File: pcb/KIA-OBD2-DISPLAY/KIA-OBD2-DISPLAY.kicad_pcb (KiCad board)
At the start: 2 copper layers, 132.1 x 19 mm, 13 parts, among them J1 Conn_01x07_Pin, U10 MCP2515-xST, U11 MCP2515-xST, U4 CAP1188-1-CP-TR, U6 TJA1050, U7 TJA1050, U9 ESP32-C6-MINI-1/U, Y1 Crystal_GND24_Small, Y4 Crystal_GND24_Small

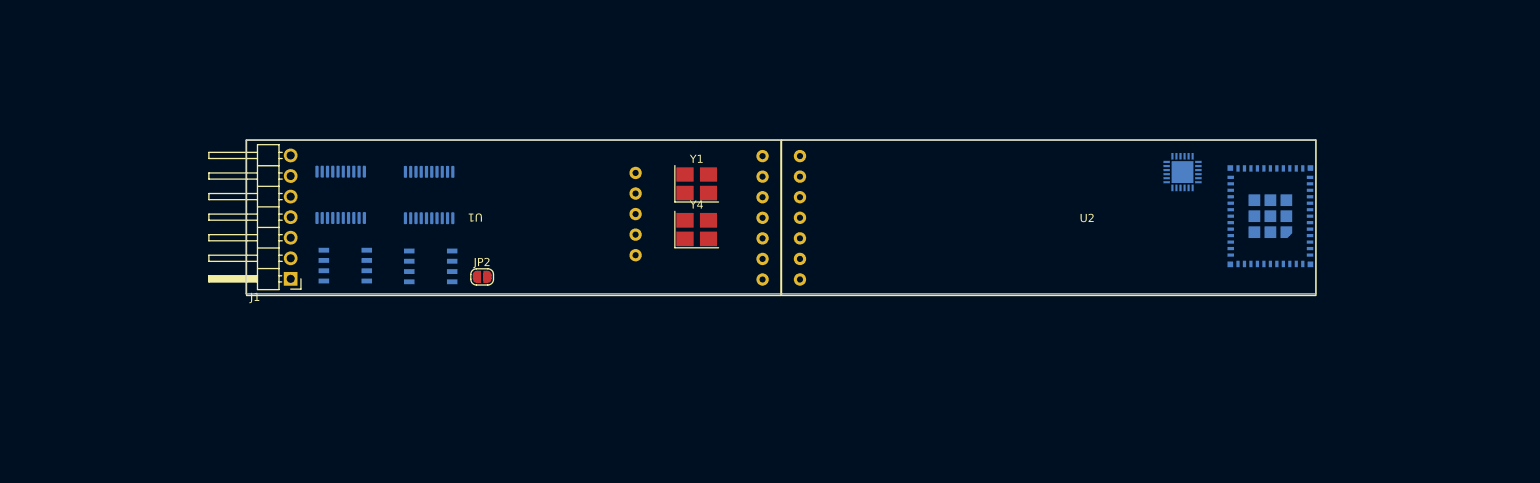
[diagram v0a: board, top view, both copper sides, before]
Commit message: pcb work
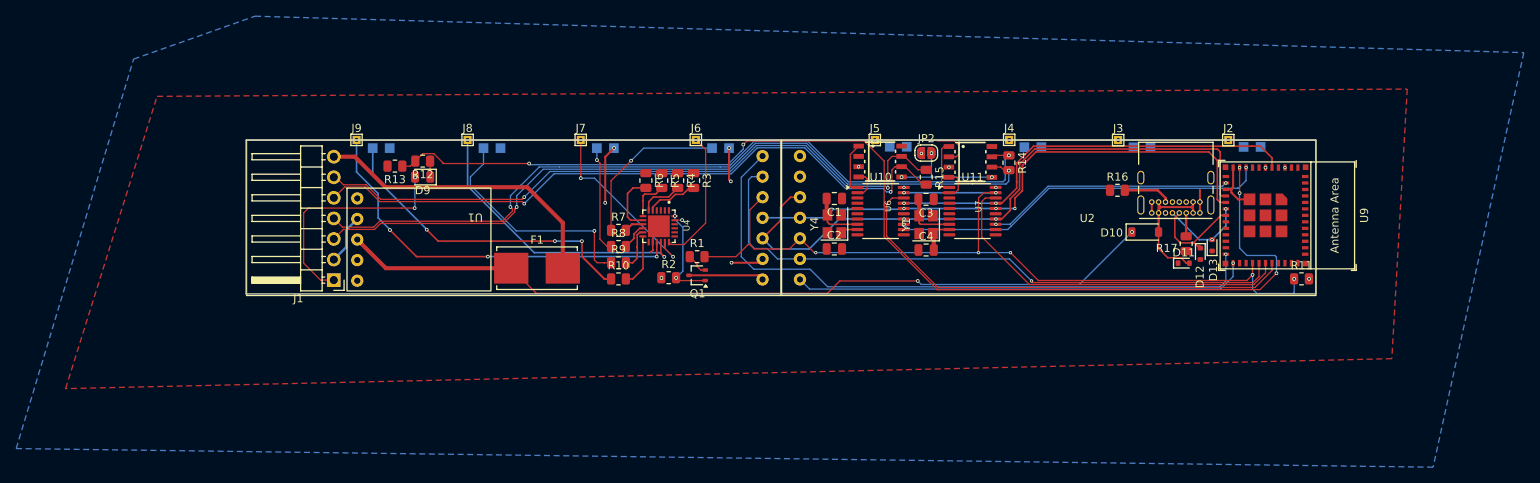
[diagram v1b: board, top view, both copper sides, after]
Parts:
- added C1: 22pF, Capacitor_SMD:C_0805_2012Metric, F.Cu at (165.9, 85.2)
- added C2: 22pF, Capacitor_SMD:C_0805_2012Metric, F.Cu at (165.9, 91.5)
- added C3: 22pF, Capacitor_SMD:C_0805_2012Metric, F.Cu at (177.3, 85.3)
- added C4: 22pF, Capacitor_SMD:C_0805_2012Metric, F.Cu at (177.3, 91.6)
- added D1: LED, LED_0602:LED_QBLP617-IW, B.Cu at (217.5, 78.8)
- added D10: 1N5819HW-7-F, Diode_SMD:D_SOD-123, F.Cu at (204.3, 89.4)
- added D11: SD05_SOD323, Diode_SMD:D_SOD-523, F.Cu at (209.1, 93.2)
- added D12: SD05_SOD323, Diode_SMD:D_SOD-523, F.Cu at (212.6, 91.0)
- added D13: STS521050B331-EA, Diode_SMD:D_SOD-523, F.Cu at (211.2, 92.0)
- added D2: LED, LED_0602:LED_QBLP617-IW, B.Cu at (203.9, 78.9)
- added D3: LED, LED_0602:LED_QBLP617-IW, B.Cu at (190.5, 78.9)
- added D4: LED, LED_0602:LED_QBLP617-IW, B.Cu at (173.8, 78.8)
- added D5: LED, LED_0602:LED_QBLP617-IW, B.Cu at (151.9, 79.0)
- added D6: LED, LED_0602:LED_QBLP617-IW, B.Cu at (137.7, 79.0)
- added D7: LED, LED_0602:LED_QBLP617-IW, B.Cu at (123.7, 79.0)
- added D8: LED, LED_0602:LED_QBLP617-IW, B.Cu at (110.0, 79.0)
- added D9: D, Diode_SMD:D_0805_2012Metric, F.Cu at (115.1, 82.6)
- added F1: Fuse_Small, Fuse:Fuseholder_Littelfuse_Nano2_154x, F.Cu at (129.2, 93.8)
- added J2: Conn_01x01, TestPoint:TestPoint_THTPad_1.0x1.0mm_Drill0.5mm, F.Cu at (214.6, 78.0)
- added J3: Conn_01x01, TestPoint:TestPoint_THTPad_1.0x1.0mm_Drill0.5mm, F.Cu at (201.0, 78.0)
- added J4: Conn_01x01, TestPoint:TestPoint_THTPad_1.0x1.0mm_Drill0.5mm, F.Cu at (187.5, 78.0)
- added J5: Conn_01x01, TestPoint:TestPoint_THTPad_1.0x1.0mm_Drill0.5mm, F.Cu at (170.9, 78.0)
- added J6: Conn_01x01, TestPoint:TestPoint_THTPad_1.0x1.0mm_Drill0.5mm, F.Cu at (148.8, 78.0)
- added J7: Conn_01x01, TestPoint:TestPoint_THTPad_1.0x1.0mm_Drill0.5mm, F.Cu at (134.6, 78.0)
- added J8: Conn_01x01, TestPoint:TestPoint_THTPad_1.0x1.0mm_Drill0.5mm, F.Cu at (120.7, 78.0)
- added J9: Conn_01x01, TestPoint:TestPoint_THTPad_1.0x1.0mm_Drill0.5mm, F.Cu at (106.9, 78.0)
- added P1: USB_C_Plug, Connector_USB:USB_C_Receptacle_GCT_USB4085, F.Cu at (211.1, 87.0)
- added Q1: BC817, Package_TO_SOT_SMD:SOT-323_SC-70, F.Cu at (149.0, 94.7)
- added R1: R, Resistor_SMD:R_0805_2012Metric, F.Cu at (149.0, 92.4)
- added R10: R, Resistor_SMD:R_0805_2012Metric, F.Cu at (139.3, 95.2)
- added R11: R, Resistor_SMD:R_0805_2012Metric, F.Cu at (223.6, 95.1)
- added R12: R, Resistor_SMD:R_0805_2012Metric, F.Cu at (115.1, 80.6)
- added R13: R, Resistor_SMD:R_0805_2012Metric, F.Cu at (111.7, 81.2)
- added R14: 120R, Resistor_SMD:R_0805_2012Metric, F.Cu at (187.5, 80.8)
- added R15: 120R, Resistor_SMD:R_0805_2012Metric, F.Cu at (177.3, 82.6)
- added R16: 5.1k, Resistor_SMD:R_0805_2012Metric, F.Cu at (200.9, 84.2)
- added R17: 5.1k, Resistor_SMD:R_0805_2012Metric, F.Cu at (209.4, 90.8)
- added R2: R, Resistor_SMD:R_0805_2012Metric, F.Cu at (145.5, 95.0)
- added R3: R, Resistor_SMD:R_0805_2012Metric, F.Cu at (148.6, 83.0)
- added R4: R, Resistor_SMD:R_0805_2012Metric, F.Cu at (146.6, 83.0)
- added R5: R, Resistor_SMD:R_0805_2012Metric, F.Cu at (144.6, 83.0)
- added R6: R, Resistor_SMD:R_0805_2012Metric, F.Cu at (142.7, 83.0)
- added R7: R, Resistor_SMD:R_0805_2012Metric, F.Cu at (139.3, 89.2)
- added R8: R, Resistor_SMD:R_0805_2012Metric, F.Cu at (139.3, 91.2)
- added R9: R, Resistor_SMD:R_0805_2012Metric, F.Cu at (139.3, 93.2)
- U10, U11, U4, U6, U7, U8, U9: moved to F.Cu
- Y1, Y4: footprint Crystal:Crystal_SMD_3225-4Pin_3.2x2.5mm_HandSoldering -> Crystal:Crystal_SMD_3225-4Pin_3.2x2.5mm
- moved U7 78.3 mm to (182.8, 80.7)
- moved U11 78.1 mm to (183.0, 86.8), turned to 0 degrees
- moved U4 65.0 mm to (144.3, 88.6), turned to -90 degrees
- moved U6 57.0 mm to (171.6, 80.7)
- moved JP2 56.9 mm to (177.3, 79.6)
- moved U10 55.8 mm to (171.7, 86.8), turned to 0 degrees
- moved U8 37.0 mm to (105.8, 83.9), turned to 0 degrees
- moved Y1 28.8 mm to (177.3, 88.5), turned to 90 degrees
- moved Y4 17.0 mm to (165.9, 88.3), turned to 90 degrees
- moved J1 5.33 mm to (104.1, 95.3)
- moved U9 0.61 mm to (221.9, 87.3), turned to -90 degrees
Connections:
- U10 pad 9: GND -> Net-(U10-OSC1)
- U4 pad 15: unconnected-(U4-CS8-Pad15) -> Net-(J9-Pin_1)
- U4 pad 16: unconnected-(U4-CS7-Pad16) -> Net-(J8-Pin_1)
- U4 pad 17: unconnected-(U4-CS6-Pad17) -> Net-(J7-Pin_1)
- U4 pad 18: unconnected-(U4-CS5-Pad18) -> Net-(J6-Pin_1)
- U4 pad 19: unconnected-(U4-CS4-Pad19) -> Net-(J5-Pin_1)
- U4 pad 20: unconnected-(U4-CS3-Pad20) -> Net-(J4-Pin_1)
- U4 pad 21: unconnected-(U4-CS2-Pad21) -> Net-(J3-Pin_1)
- U4 pad 22: unconnected-(U4-CS1-Pad22) -> Net-(J2-Pin_1)
- U9 pad 17: unconnected-(U9-GPIO12/USB_D--Pad17) -> Net-(D12-A2)
- U9 pad 18: unconnected-(U9-GPIO13/USB_D+-Pad18) -> Net-(D13-A1)
- Y4 pad 1: GND -> Net-(U10-OSC1)
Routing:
- net /INTING: track 0.00 -> 141.7 mm, vias 0 -> 5
- net /REST: track 0.00 -> 108.9 mm, vias 0 -> 7
- net +12V: track 0.00 -> 102.0 mm, vias 0 -> 2
- net /CAN LISTEN H: track 0.00 -> 97.2 mm, vias 0 -> 2
- net /CAN LISTEN L: track 0.00 -> 95.2 mm, vias 0 -> 2
- net /OBD2 CAN H: track 0.00 -> 83.6 mm, vias 0 -> 2
- net /OBD2 CAN L: track 0.00 -> 83.4 mm, vias 0 -> 2
- net /SCLK: track 0.00 -> 78.7 mm, vias 0 -> 2
- net /CSD1: track 0.00 -> 78.5 mm, vias 0 -> 1
- net /DC: track 0.00 -> 76.7 mm, vias 0 -> 1
- net /MOSI: track 0.00 -> 69.3 mm, vias 0 -> 3
- net /CSCAN: track 0.00 -> 58.4 mm
- net /CSD2: track 0.00 -> 56.3 mm, vias 0 -> 1
- net /MISO: track 0.00 -> 52.0 mm, vias 0 -> 2
- net Net-(J9-Pin_1): track 0.00 -> 48.8 mm, vias 0 -> 3
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- added copper zone on B.Cu, net +3.3V
- added copper zone on F.Cu, net GND
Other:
- outline, holes or cut-outs redrawn
